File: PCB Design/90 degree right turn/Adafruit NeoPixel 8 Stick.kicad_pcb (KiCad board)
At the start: 2 copper layers, 24.4 x 23.9 mm, 5 parts, among them CN1 1X4SMT, CN2 1X4SMT

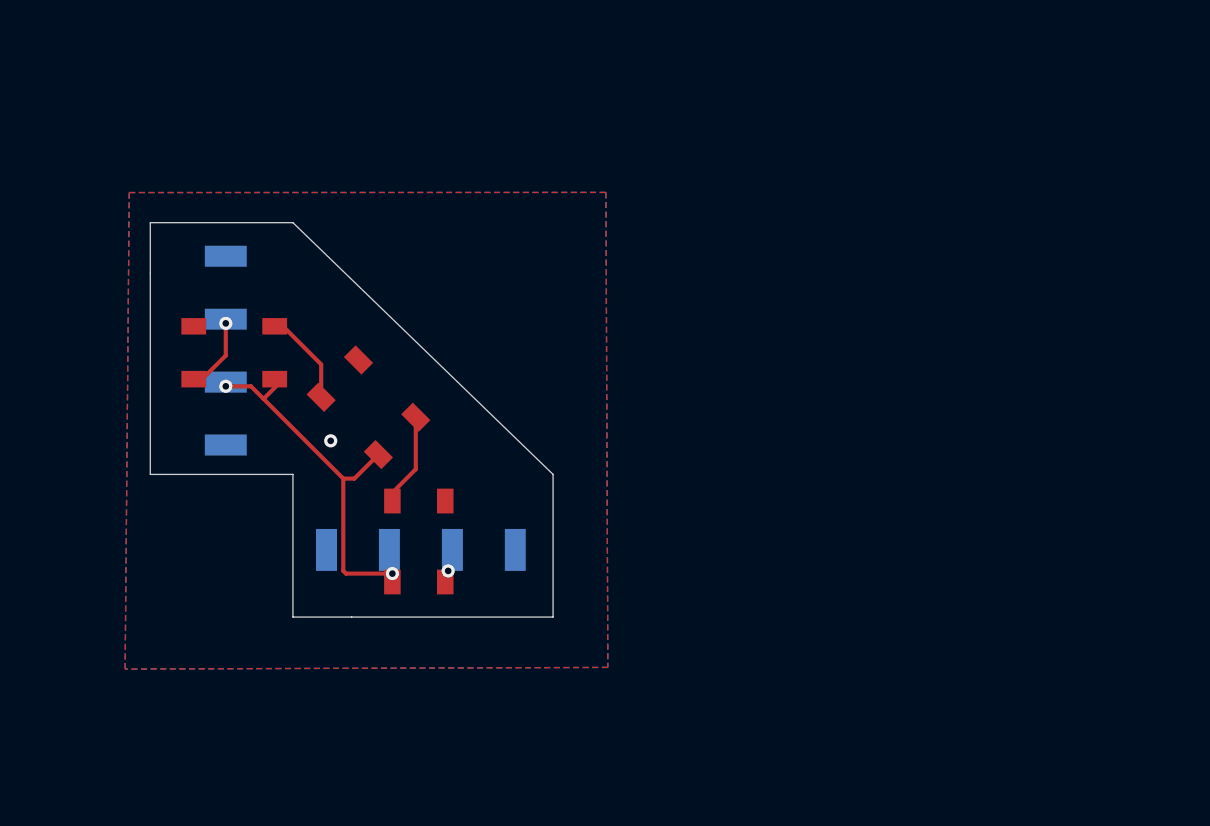
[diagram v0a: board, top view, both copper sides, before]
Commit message: 6 pin
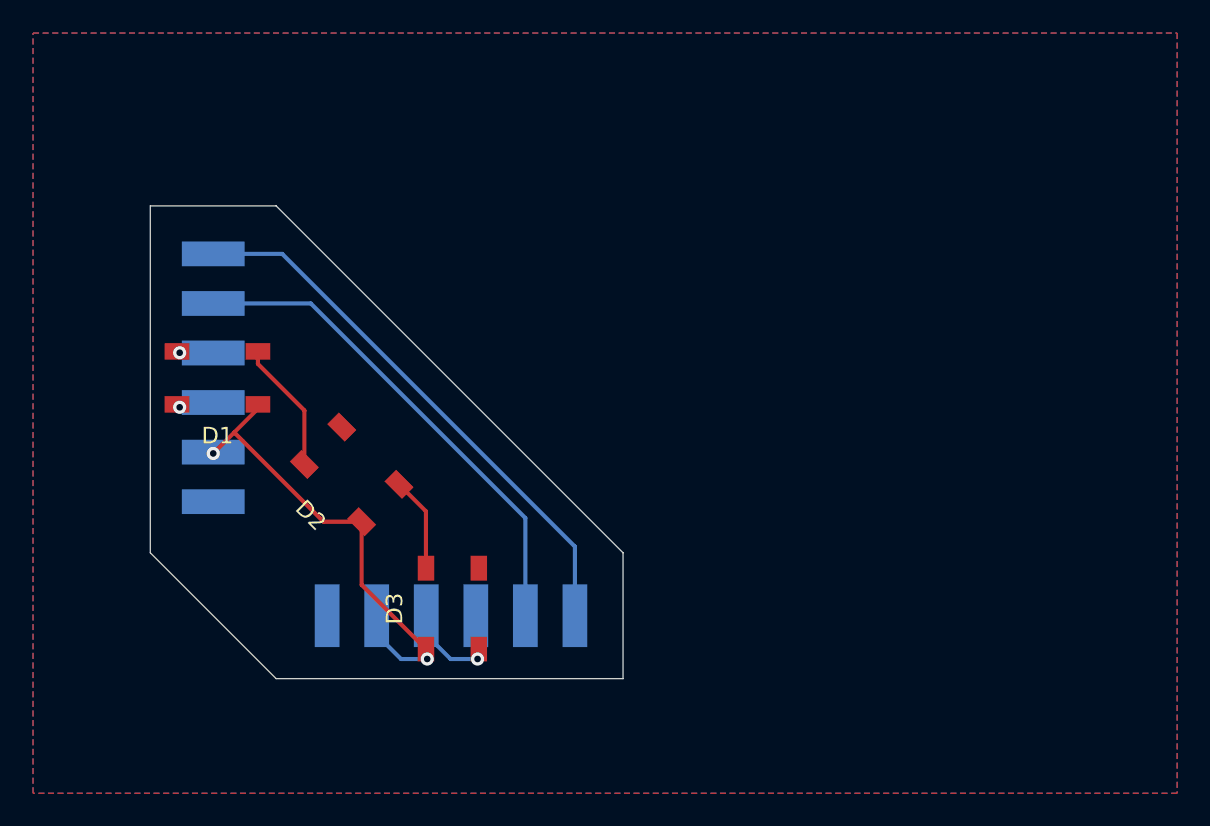
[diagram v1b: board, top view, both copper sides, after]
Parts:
- moved D3 4.54 mm to (140.7, 121.9)
- moved D2 4.19 mm to (134.6, 113.8)
- moved CN1 3.42 mm to (140.1, 121.7)
- moved D1 1.83 mm to (126.5, 108.0)
- moved CN2 0.52 mm to (126.9, 107.4)
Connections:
- CN1 pad 1: GND -> Net-(CN1-Pad1)
- CN1 pad 3: +5V -> GND
- CN1 pad 4: GND -> Net-(D3-Pad2)
- D3 pad 2: Net-(CN1-Pad2) -> Net-(D3-Pad2)
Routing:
- net Net-(CN1-Pad1): track 0.00 -> 33.4 mm
- net Net-(CN1-Pad2): track 0.00 -> 30.2 mm, vias 1 -> 0
- net +5V: track 22.5 -> 28.2 mm
- net Net-(D3-Pad2): track 0.00 -> 4.87 mm, vias 0 -> 1
- net Net-(CN2-Pad3): track 3.97 -> 0.00 mm
- net Net-(D1-Pad2): track 5.26 -> 8.01 mm
- net Net-(D2-Pad2): track 5.16 -> 5.75 mm
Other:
- board size 24.4 x 23.9 mm -> 28.6 x 28.6 mm
- board text removed: "4-7VDC"
- board text removed: "DOUT"
- board text removed: "GND"
